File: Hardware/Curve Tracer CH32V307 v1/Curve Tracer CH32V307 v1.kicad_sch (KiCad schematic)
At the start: 66 parts, among them J1 To CH32V307V-ETH, J2 Probes, J3 Power Supply, U1 OPA356xxDBV, U10 MAX393, U11 ICL7660, U12 LM7805_TO220, U2 AMS1117-3.3, U3 USBLC6-4SC6, U4 OPA356xxDBV, U5 OPA356xxDBV, U6 OPA356xxDBV, U7 MAX393, U8 MAX393, U9 MAX393

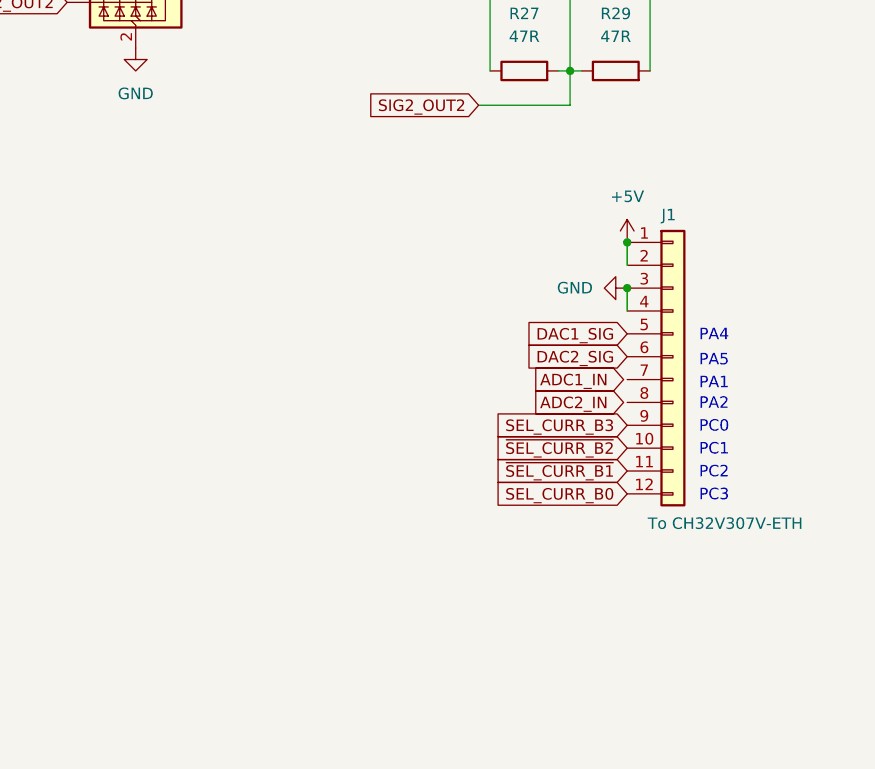
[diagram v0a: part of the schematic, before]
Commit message: Update
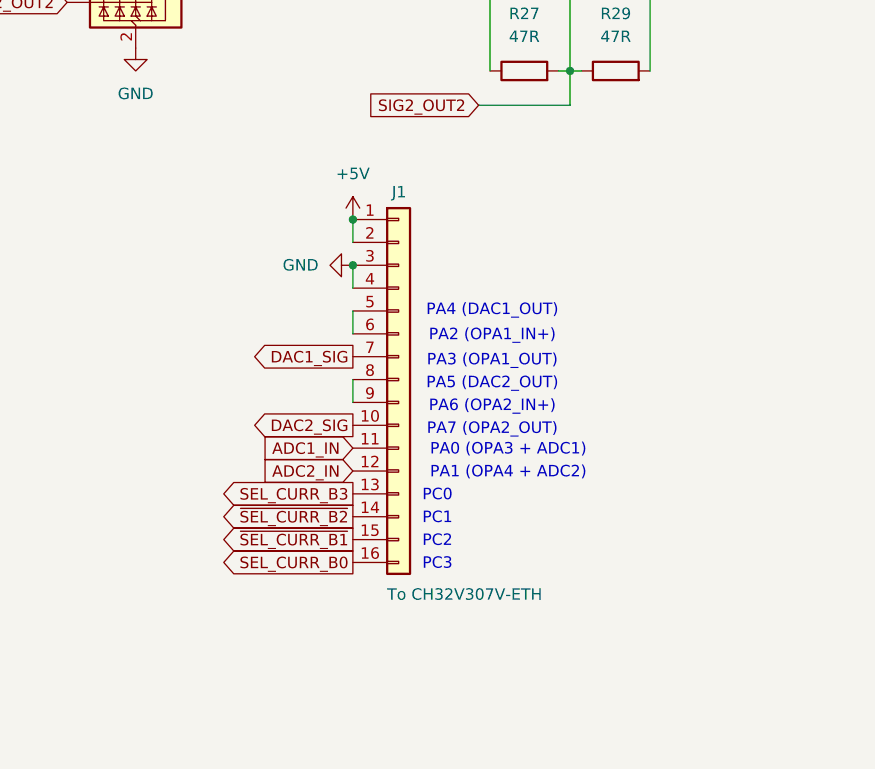
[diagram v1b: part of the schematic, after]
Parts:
- removed J1: To CH32V307V-ETH, symbol Connector_Generic:Conn_01x12
- added J1: To CH32V307V-ETH, symbol Connector_Generic:Conn_01x16
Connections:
- net +5V: now also J1.1 (Pin_1), J1.2 (Pin_2)
- net ADC1_IN: now also J1.11 (Pin_11)
- net ADC2_IN: now also J1.12 (Pin_12)
- net DAC1_SIG: now also J1.7 (Pin_7)
- net DAC2_SIG: now also J1.10 (Pin_10)
- net GND: now also J1.3 (Pin_3), J1.4 (Pin_4)
- net SEL_CURR_B0: now also J1.16 (Pin_16)
- net SEL_CURR_B3: now also J1.13 (Pin_13)
- net ~{SEL_CURR_B1}: now also J1.15 (Pin_15)
- net ~{SEL_CURR_B2}: now also J1.14 (Pin_14)
- new net: J1.5 (Pin_5), J1.6 (Pin_6)
- new net: J1.8 (Pin_8), J1.9 (Pin_9)
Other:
- note added: "PA0 (OPA3 + ADC1)"
- note added: "PA1 (OPA4 + ADC2)"
- note added: "PA2 (OPA1_IN+)"
- note added: "PA3 (OPA1_OUT)"
- note added: "PA4 (DAC1_OUT)"
- note added: "PA5 (DAC2_OUT)"
- note added: "PA6 (OPA2_IN+)"
- note added: "PA7 (OPA2_OUT)"
- note removed: "PA1"
- note removed: "PA2"
- note removed: "PA4"
- note removed: "PA5"
